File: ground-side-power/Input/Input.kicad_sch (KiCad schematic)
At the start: 32 parts, among them J1 Battery Terminals, J2 Battery Terminals, J26 Conn_01x02_Female, J5 874270842, J6 874270842, J7 ATX-24, K1 AZ2150-1A-12DEF, K3 AZ2150-1A-12DEF, M1 Fan_PC_Chassis, U1 INA180, U2 INA180

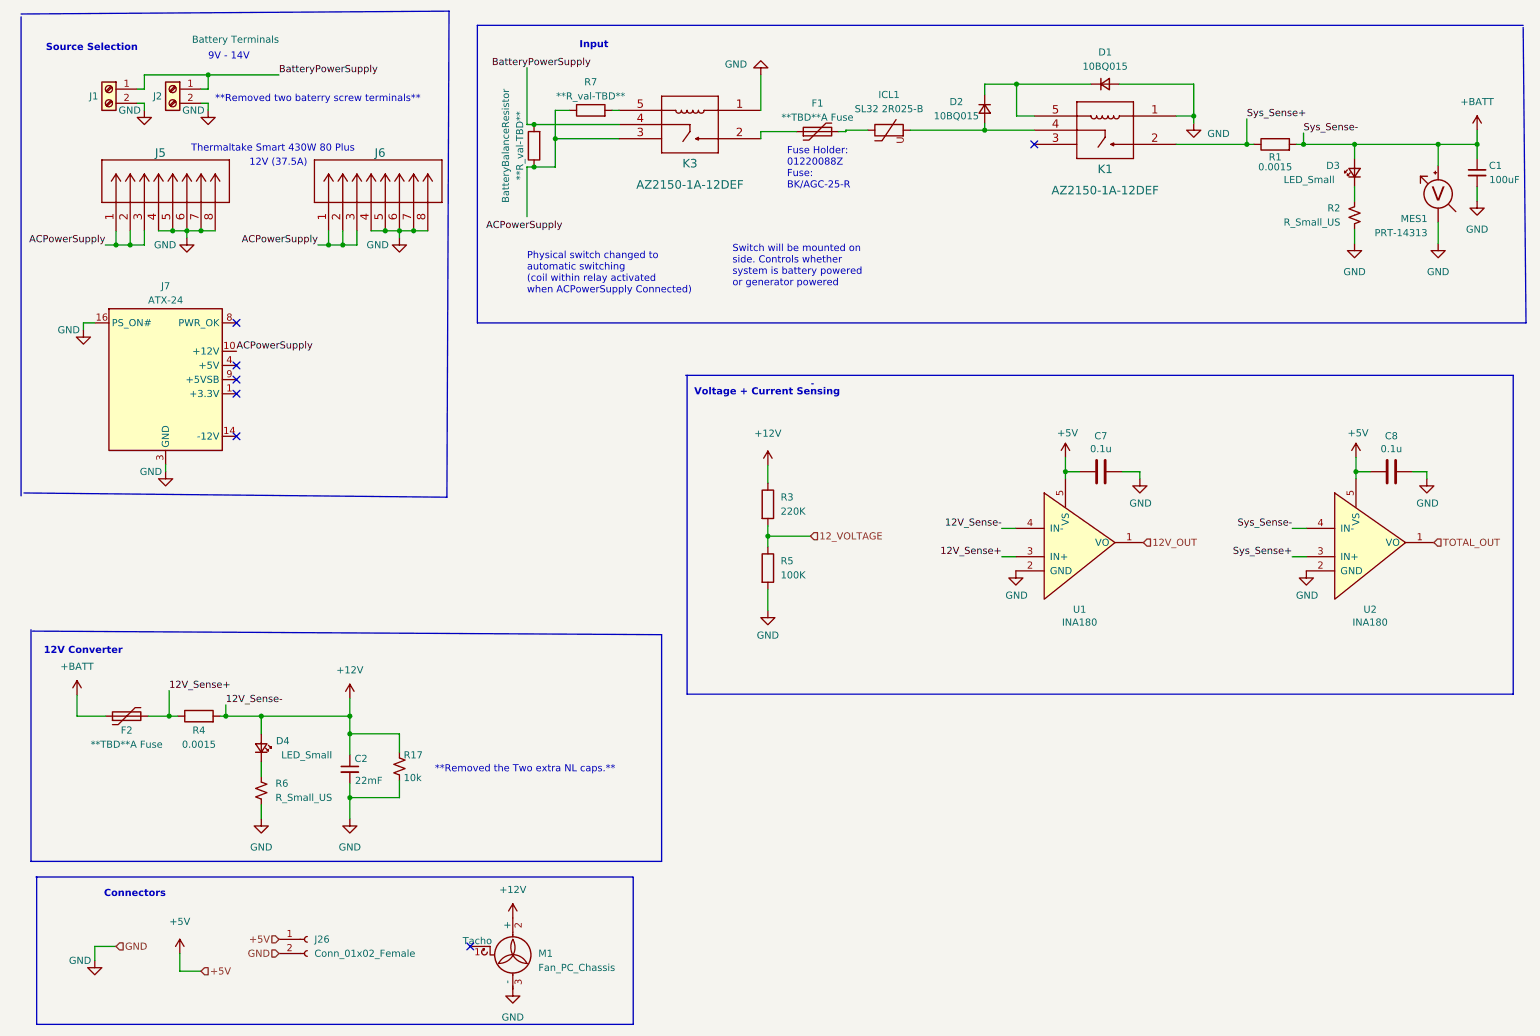
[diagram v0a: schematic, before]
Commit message: New changes from Review
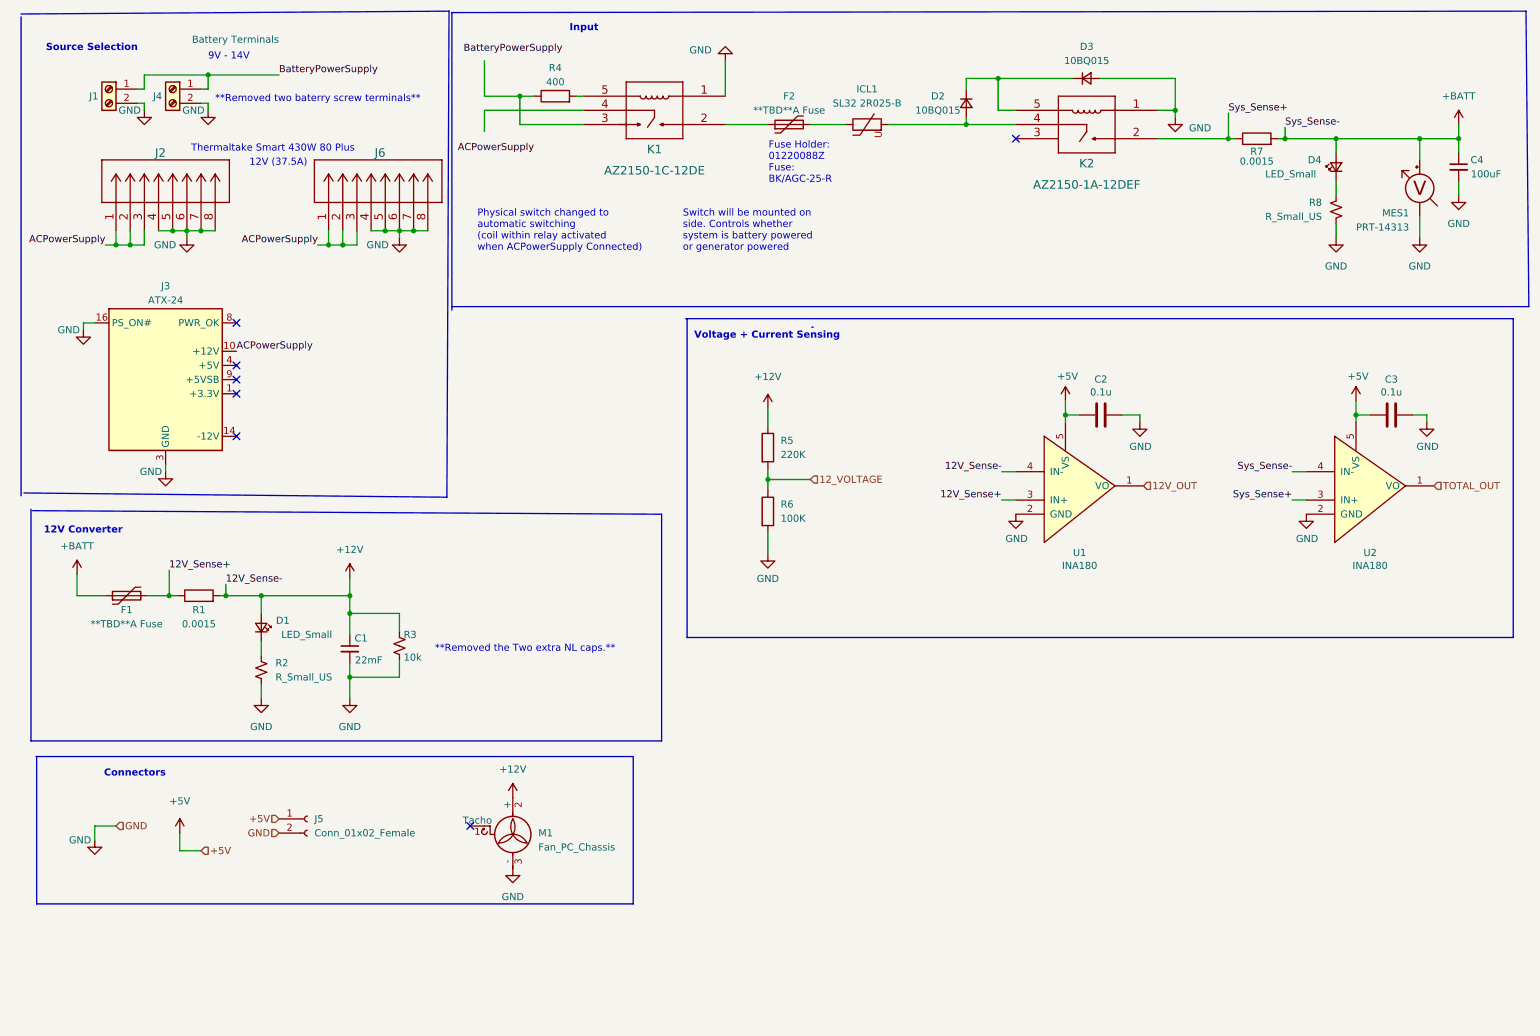
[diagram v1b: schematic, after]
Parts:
- removed BatteryBalanceResistor: **R_val-TBD**, Resistor_SMD:R_0805_2012Metric_Pad1.20x1.40mm_HandSolder, symbol Device:R
- K1: renamed from K3; value AZ2150-1A-12DEF -> AZ2150-1C-12DE
- R4: renamed from R7; value **R_val-TBD** -> 400
- renumbered C2 to C1, C7 to C2, C8 to C3, C1 to C4, D4 to D1, D1 to D3, D3 to D4, F2 to F1, F1 to F2, J5 to J2, J7 to J3, J2 to J4, J26 to J5, K1 to K2, R4 to R1, R6 to R2, R17 to R3, R3 to R5, R5 to R6, R1 to R7, R2 to R8
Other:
- moved on the sheet: C1, C2, C3, C4, D1, D2, D3, D4, F1, F2, ICL1, J5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
